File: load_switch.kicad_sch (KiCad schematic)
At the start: 8 parts, among them U2 XC6192B

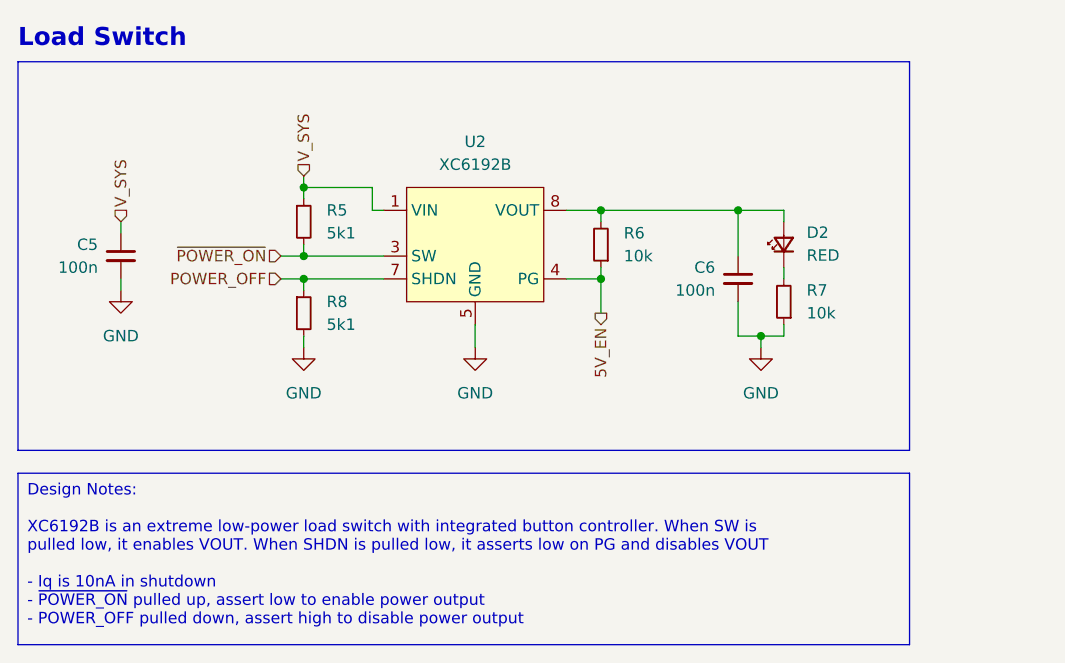
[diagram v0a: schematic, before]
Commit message: finish all schematic changes
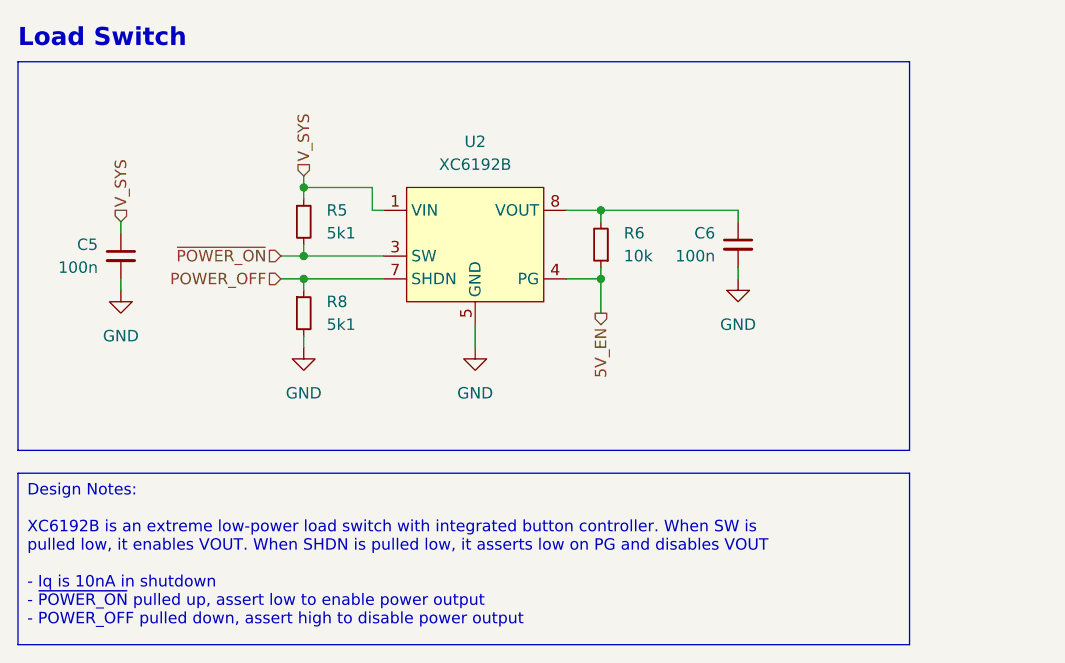
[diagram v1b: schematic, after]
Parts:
- removed D2: RED, LED_SMD:LED_0402_1005Metric, symbol Device:LED_Small
- removed R7: 10k, Resistor_SMD:R_0402_1005Metric, symbol Device:R_Small
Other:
- moved on the sheet: C6
